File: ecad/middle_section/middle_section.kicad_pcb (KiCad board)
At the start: 2 copper layers, 100 x 80 mm, 36 parts, among them J1 JST SH, J2 JST SH 6P, J3 Micro-MaTch 2x06, U1 ATtiny1617-M

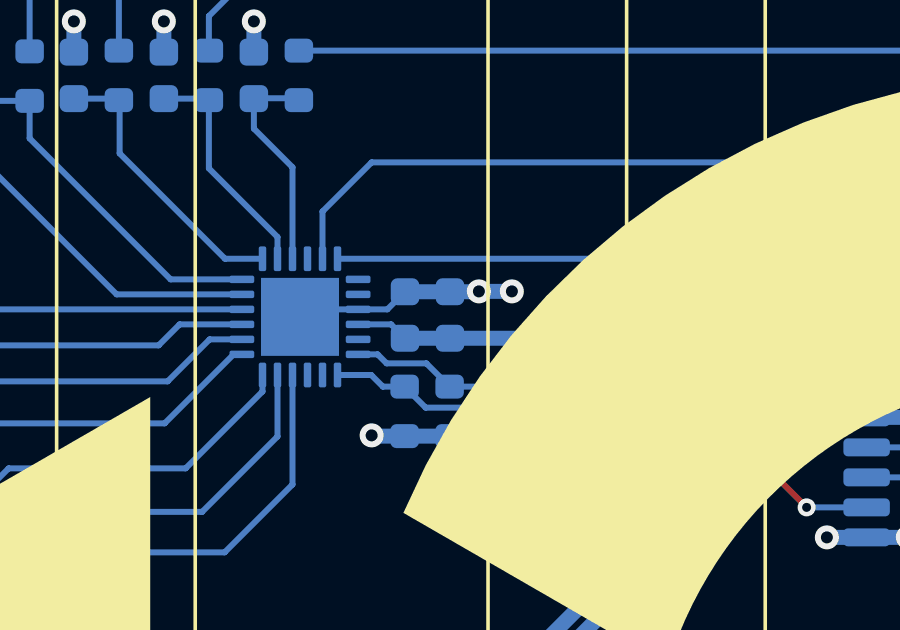
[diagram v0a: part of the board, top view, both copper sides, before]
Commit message: First production run for PCB
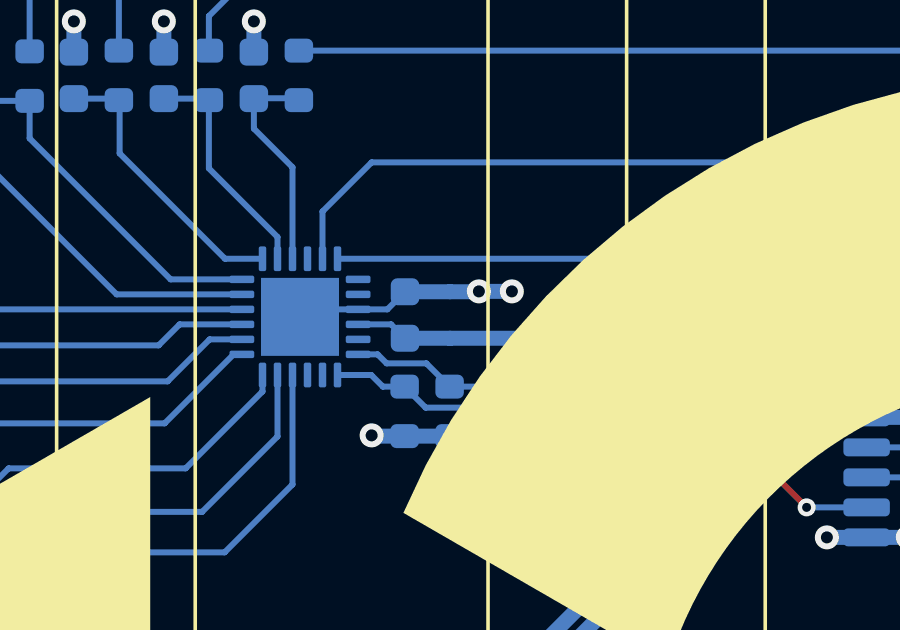
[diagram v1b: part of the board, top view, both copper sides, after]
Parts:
- removed C4: 10u, Capacitor_SMD:C_0603_1608Metric
- J2: footprint Connector_JST:JST_SH_SM06B-SRSS-TB_1x06-1MP_P1.00mm_Horizontal -> woodpecker:JST_SH_SM06B-SRSS-TB_1x06-1MP_P1.00mm_Horizontal
- R6, R7: value 10k -> 33k
